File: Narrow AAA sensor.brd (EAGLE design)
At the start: 42.7 x 10.8 mm, 16 parts, among them IC1 LD117AS33TR, U1 ATMEGA328P_PDIP

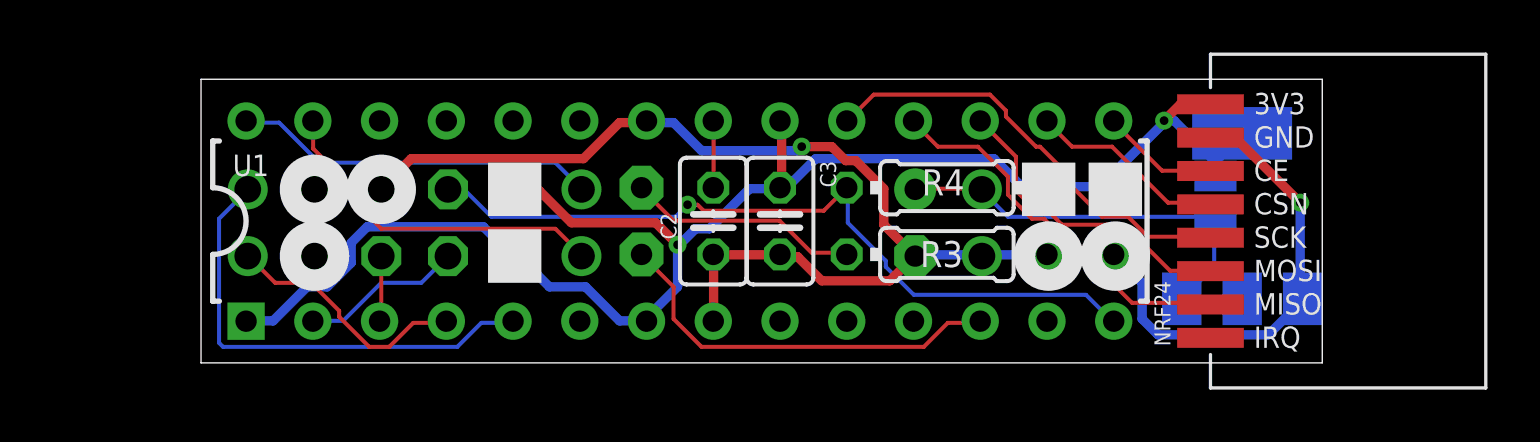
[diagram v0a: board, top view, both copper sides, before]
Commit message: https://PCBs.io/share/zM3DO
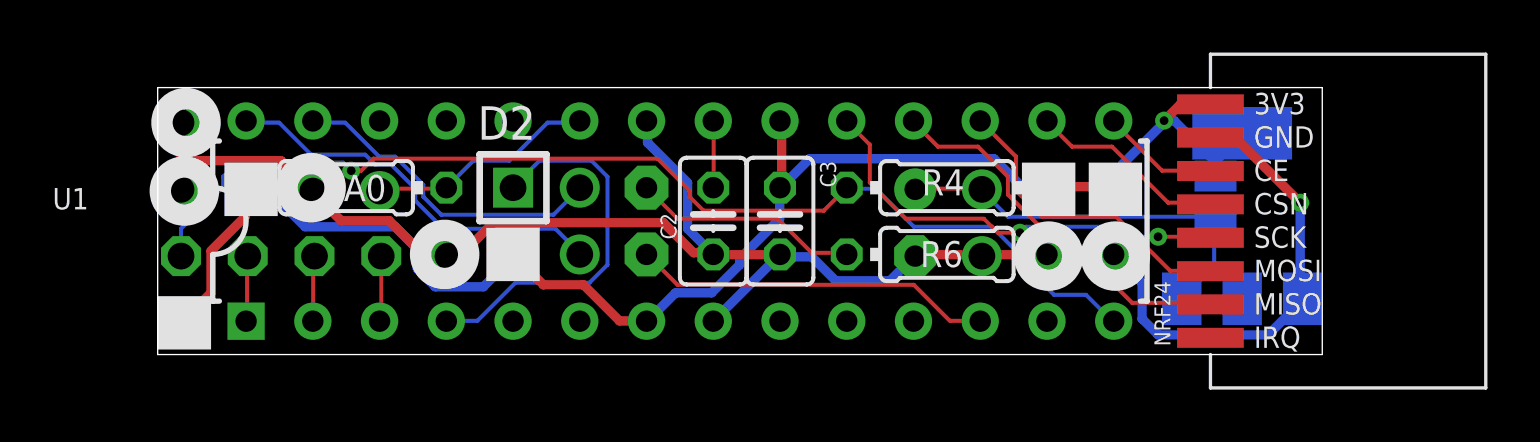
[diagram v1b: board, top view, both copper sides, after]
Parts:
- removed J2: (no value), SparkFun-Connectors:1X02
- removed SENSOR: (no value), pinhead:1X04
- added A0-GND: Analog, SparkFun-Connectors:1X02
- added D2: (no value), pinhead:1X01
- added RA0: 10K, rcl:0204/7
- added VCC-D-GND-GND: Sensor, pinhead:1X04
- SERIAL: device pinhead:1X04 -> pinhead:1X05
- moved J3 2.60 mm to (17.5, 6.67), turned to 270 degrees
- moved SERIAL 1.27 mm to (9.91, 4.06)
- moved LED1 0.19 mm to (20.0, 5.40)
- renumbered R3 to R6
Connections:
- removed net A1: U1.24
- removed net D3: J2.2, U1.5
- new net RESET: SERIAL.5, U1.1
- net A0: now also A0-GND.1, RA0.1
- net D2: now also D2.1; no longer J2.1
- net GND: now also A0-GND.2, SERIAL.2, VCC-D-GND-GND.3, VCC-D-GND-GND.4; no longer SENSOR.3, SENSOR.4, SERIAL.4
- net RXD: now also SERIAL.4; no longer SERIAL.2
- net TMP: now also VCC-D-GND-GND.2; no longer SENSOR.2
- net VCC: now also RA0.2, VCC-D-GND-GND.1; no longer SENSOR.1, U1.1
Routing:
- net D3: track 17.9 -> 0.00 mm
- net TMP: track 29.4 -> 41.7 mm
- net A0: track 0.00 -> 8.75 mm
- net D2: track 9.53 -> 14.7 mm
- net RXD: track 6.17 -> 2.51 mm
- net GND: track 66.3 -> 69.2 mm, vias 2 -> 1
- net RESET: track 0.00 -> 2.51 mm
- net D6: track 15.5 -> 13.7 mm
- net SCL: track 13.9 -> 15.1 mm
- net VCC: track 61.5 -> 60.5 mm, vias 2 -> 1
- net SDA: track 13.3 -> 12.4 mm
- net SCK: track 16.8 -> 16.7 mm, vias 0 -> 2
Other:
- board size 42.7 x 10.8 mm -> 44.3 x 10.2 mm
- board text removed: "D2"
- board text removed: "D3"
